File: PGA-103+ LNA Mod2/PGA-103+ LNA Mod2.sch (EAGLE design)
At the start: 42 parts, among them IC1 7805DT, K1 G2RE, K2 G2RE, K3 G2RE, K4 G2RE, X1 SMA, X2 SMA

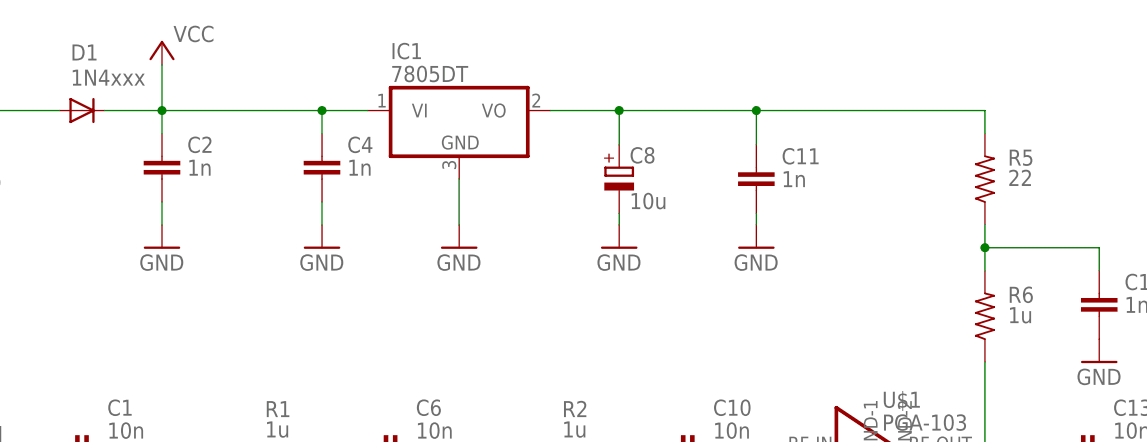
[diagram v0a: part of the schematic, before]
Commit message: First commit
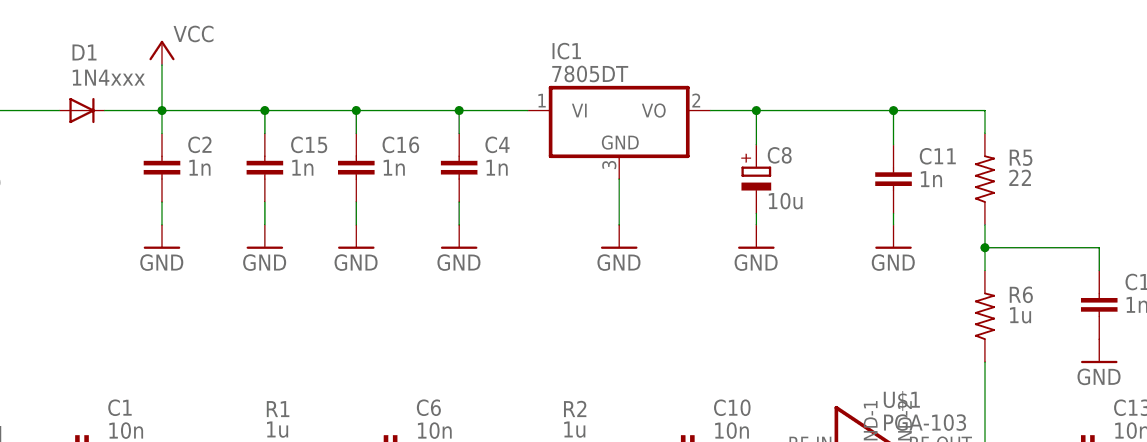
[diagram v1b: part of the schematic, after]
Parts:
- added C15, C16: 1n, rcl:C-EUC1206
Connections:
- net GND: now also C15.2, C16.2
- net VCC: now also C15.1, C16.1
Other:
- moved on the sheet: C11, C4, C8, IC1
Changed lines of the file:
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@@
 <part name="C8" library="rcl" deviceset="CPOL-EU" device="B/3528-21R" value="10u"/>
 <part name="U$1" library="minicircuits" deviceset="PGA-103" device=""/>
+<part name="GND23" library="supply1" deviceset="GND" device=""/>
+<part name="C15" library="rcl" deviceset="C-EU" device="C1206" value="1n"/>
+<part name="GND24" library="supply1" deviceset="GND" device=""/>
+<part name="C16" library="rcl" deviceset="C-EU" device="C1206" value="1n"/>
 </parts>
 <sheets>
@@
 <attribute name="VALUE" x="82.804" y="37.211" size="1.778" layer="96"/>
 </instance>
-<instance part="C11" gate="G$1" x="80.01" y="96.52" smashed="yes">
-<attribute name="NAME" x="82.804" y="96.901" size="1.778" layer="95"/>
-<attribute name="VALUE" x="82.804" y="94.361" size="1.778" layer="96"/>
+<instance part="C11" gate="G$1" x="95.25" y="96.52" smashed="yes">
+<attribute name="NAME" x="98.044" y="96.901" size="1.778" layer="95"/>
+<attribute name="VALUE" x="98.044" y="94.361" size="1.778" layer="96"/>
 </instance>
 <instance part="C14" gate="G$1" x="118.11" y="80.01" smashed="yes" rot="R180">
@@
 </instance>
 <instance part="GND17" gate="1" x="92.71" y="52.07"/>
-<instance part="GND9" gate="1" x="46.99" y="87.63"/>
-<instance part="GND6" gate="1" x="31.75" y="87.63"/>
-<instance part="GND12" gate="1" x="64.77" y="87.63"/>
-<instance part="GND14" gate="1" x="80.01" y="87.63"/>
+<instance part="GND9" gate="1" x="64.77" y="87.63"/>
+<instance part="GND6" gate="1" x="46.99" y="87.63"/>
+<instance part="GND12" gate="1" x="80.01" y="87.63"/>
+<instance part="GND14" gate="1" x="95.25" y="87.63"/>
 <instance part="R6" gate="G$1" x="105.41" y="80.01" smashed="yes" rot="R90">
 <attribute name="NAME" x="107.95" y="81.5086" size="1.778" layer="95"/>
@@
 <instance part="GND2" gate="1" x="-6.35" y="5.08"/>
 <instance part="X1" gate="G1" x="-8.89" y="12.7"/>
-<instance part="C4" gate="G$1" x="31.75" y="97.79" smashed="yes">
-<attribute name="NAME" x="34.544" y="98.171" size="1.778" layer="95"/>
-<attribute name="VALUE" x="34.544" y="95.631" size="1.778" layer="96"/>
+<instance part="C4" gate="G$1" x="46.99" y="97.79" smashed="yes">
+<attribute name="NAME" x="49.784" y="98.171" size="1.778" layer="95"/>
+<attribute name="VALUE" x="49.784" y="95.631" size="1.778" layer="96"/>
 </instance>
 <instance part="C2" gate="G$1" x="13.97" y="97.79" smashed="yes">
@@
 </instance>
 <instance part="GND4" gate="1" x="13.97" y="87.63"/>
-<instance part="IC1" gate="A1" x="46.99" y="102.87"/>
+<instance part="IC1" gate="A1" x="64.77" y="102.87"/>
 <instance part="C1" gate="G$1" x="3.81" y="64.77" smashed="yes" rot="R90">
 <attribute name="NAME" x="7.874" y="68.961" size="1.778" layer="95"/>
@@
 <instance part="L4" gate="G$1" x="147.32" y="24.13" rot="R90"/>
 <instance part="L3" gate="G$1" x="143.51" y="11.43" rot="R90"/>
-<instance part="C8" gate="G$1" x="64.77" y="96.52"/>
+<instance part="C8" gate="G$1" x="80.01" y="96.52"/>
 <instance part="U$1" gate="G$1" x="91.44" y="64.77"/>
+<instance part="GND23" gate="1" x="25.4" y="87.63"/>
+<instance part="C15" gate="G$1" x="25.4" y="97.79" smashed="yes">
+<attribute name="NAME" x="28.194" y="98.171" size="1.778" layer="95"/>
+<attribute name="VALUE" x="28.194" y="95.631" size="1.778" layer="96"/>
+</instance>
+<instance part="GND24" gate="1" x="35.56" y="87.63"/>
+<instance part="C16" gate="G$1" x="35.56" y="97.79" smashed="yes">
+<attribute name="NAME" x="38.354" y="98.171" size="1.778" layer="95"/>
+<attribute name="VALUE" x="38.354" y="95.631" size="1.778" layer="96"/>
+</instance>
 </instances>
 <busses>
@@
 <segment>
 <pinref part="GND6" gate="1" pin="GND"/>
-<wire x1="31.75" y1="90.17" x2="31.75" y2="92.71" width="0.1524" layer="91"/>
+<wire x1="46.99" y1="90.17" x2="46.99" y2="92.71" width="0.1524" layer="91"/>
 <pinref part="C4" gate="G$1" pin="2"/>
 </segment>
 <segment>
 <pinref part="GND12" gate="1" pin="GND"/>
-<wire x1="64.77" y1="90.17" x2="64.77" y2="91.44" width="0.1524" layer="91"/>
+<wire x1="80.01" y1="90.17" x2="80.01" y2="91.44" width="0.1524" layer="91"/>
 <pinref part="C8" gate="G$1" pin="-"/>
 </segment>
@@
 <pinref part="C11" gate="G$1" pin="2"/>
 <pinref part="GND14" gate="1" pin="GND"/>
-<wire x1="80.01" y1="90.17" x2="80.01" y2="91.44" width="0.1524" layer="91"/>
+<wire x1="95.25" y1="90.17" x2="95.25" y2="91.44" width="0.1524" layer="91"/>
 </segment>
 <segment>
@@
 <pinref part="IC1" gate="A1" pin="GND"/>
 <pinref part="GND9" gate="1" pin="GND"/>
-<wire x1="46.99" y1="90.17" x2="46.99" y2="95.25" width="0.1524" layer="91"/>
+<wire x1="64.77" y1="90.17" x2="64.77" y2="95.25" width="0.1524" layer="91"/>
 </segment>
 <segment>
@@
 <junction x="11.43" y="31.75"/>
 </segment>
+<segment>
+<pinref part="GND23" gate="1" pin="GND"/>
+<wire x1="25.4" y1="90.17" x2="25.4" y2="92.71" width="0.1524" layer="91"/>
+<pinref part="C15" gate="G$1" pin="2"/>
+</segment>
+<segment>
+<pinref part="GND24" gate="1" pin="GND"/>
+<wire x1="35.56" y1="90.17" x2="35.56" y2="92.71" width="0.1524" layer="91"/>
+<pinref part="C16" gate="G$1" pin="2"/>
+</segment>
 </net>
 <net name="N$5" class="0">
 <segment>
-<wire x1="57.15" y1="102.87" x2="64.77" y2="102.87" width="0.1524" layer="91"/>
-<wire x1="64.77" y1="102.87" x2="64.77" y2="99.06" width="0.1524" layer="91"/>
+<wire x1="74.93" y1="102.87" x2="80.01" y2="102.87" width="0.1524" layer="91"/>
+<wire x1="80.01" y1="102.87" x2="80.01" y2="99.06" width="0.1524" layer="91"/>
 <pinref part="R5" gate="G$1" pin="2"/>
-<wire x1="64.77" y1="102.87" x2="80.01" y2="102.87" width="0.1524" layer="91"/>
-<wire x1="80.01" y1="102.87" x2="105.41" y2="102.87" width="0.1524" layer="91"/>
+<wire x1="80.01" y1="102.87" x2="95.25" y2="102.87" width="0.1524" layer="91"/>
+<wire x1="95.25" y1="102.87" x2="105.41" y2="102.87" width="0.1524" layer="91"/>
 <wire x1="105.41" y1="102.87" x2="105.41" y2="100.33" width="0.1524" layer="91"/>
-<junction x="64.77" y="102.87"/>
+<junction x="80.01" y="102.87"/>
 <pinref part="C11" gate="G$1" pin="1"/>
-<wire x1="80.01" y1="99.06" x2="80.01" y2="102.87" width="0.1524" layer="91"/>
-<junction x="80.01" y="102.87"/>
+<wire x1="95.25" y1="99.06" x2="95.25" y2="102.87" width="0.1524" layer="91"/>
+<junction x="95.25" y="102.87"/>
 <pinref part="IC1" gate="A1" pin="VO"/>
 <pinref part="C8" gate="G$1" pin="+"/>
@@
 <net name="VCC" class="0">
 <segment>
-<wire x1="36.83" y1="102.87" x2="31.75" y2="102.87" width="0.1524" layer="91"/>
-<wire x1="31.75" y1="102.87" x2="31.75" y2="100.33" width="0.1524" layer="91"/>
+<wire x1="54.61" y1="102.87" x2="46.99" y2="102.87" width="0.1524" layer="91"/>
+<wire x1="46.99" y1="102.87" x2="46.99" y2="100.33" width="0.1524" layer="91"/>
 <pinref part="D1" gate="G$1" pin="C"/>
 <wire x1="7.62" y1="102.87" x2="13.97" y2="102.87" width="0.1524" layer="91"/>
-<junction x="31.75" y="102.87"/>
+<junction x="46.99" y="102.87"/>
 <pinref part="C4" gate="G$1" pin="1"/>
 <pinref part="IC1" gate="A1" pin="VI"/>
-<wire x1="13.97" y1="102.87" x2="31.75" y2="102.87" width="0.1524" layer="91"/>
+<wire x1="13.97" y1="102.87" x2="25.4" y2="102.87" width="0.1524" layer="91"/>
+<wire x1="25.4" y1="102.87" x2="35.56" y2="102.87" width="0.1524" layer="91"/>
+<wire x1="35.56" y1="102.87" x2="46.99" y2="102.87" width="0.1524" layer="91"/>
 <wire x1="13.97" y1="100.33" x2="13.97" y2="102.87" width="0.1524" layer="91"/>
 <junction x="13.97" y="102.87"/>
@@
 <pinref part="P+1" gate="VCC" pin="VCC"/>
 <wire x1="13.97" y1="102.87" x2="13.97" y2="107.95" width="0.1524" layer="91"/>
-</segment>
-<segment>
+<pinref part="C15" gate="G$1" pin="1"/>
+<wire x1="25.4" y1="100.33" x2="25.4" y2="102.87" width="0.1524" layer="91"/>
+<junction x="25.4" y="102.87"/>
+<pinref part="C16" gate="G$1" pin="1"/>
+<wire x1="35.56" y1="100.33" x2="35.56" y2="102.87" width="0.1524" layer="91"/>
+<junction x="35.56" y="102.87"/>
+</segment>
+<segment>
